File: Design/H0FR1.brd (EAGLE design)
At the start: 60 x 34.6 mm, 34 parts, among them P1 HEXABIT_X2_P1_P5_EDIT_POWER_P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, Q1 BSS123, U1 STM32G0B1CEU6QFN_B1CEU6_STM-L, U2 G5LE-14_DC3, X1 XTALL_CSTCE8M00G52

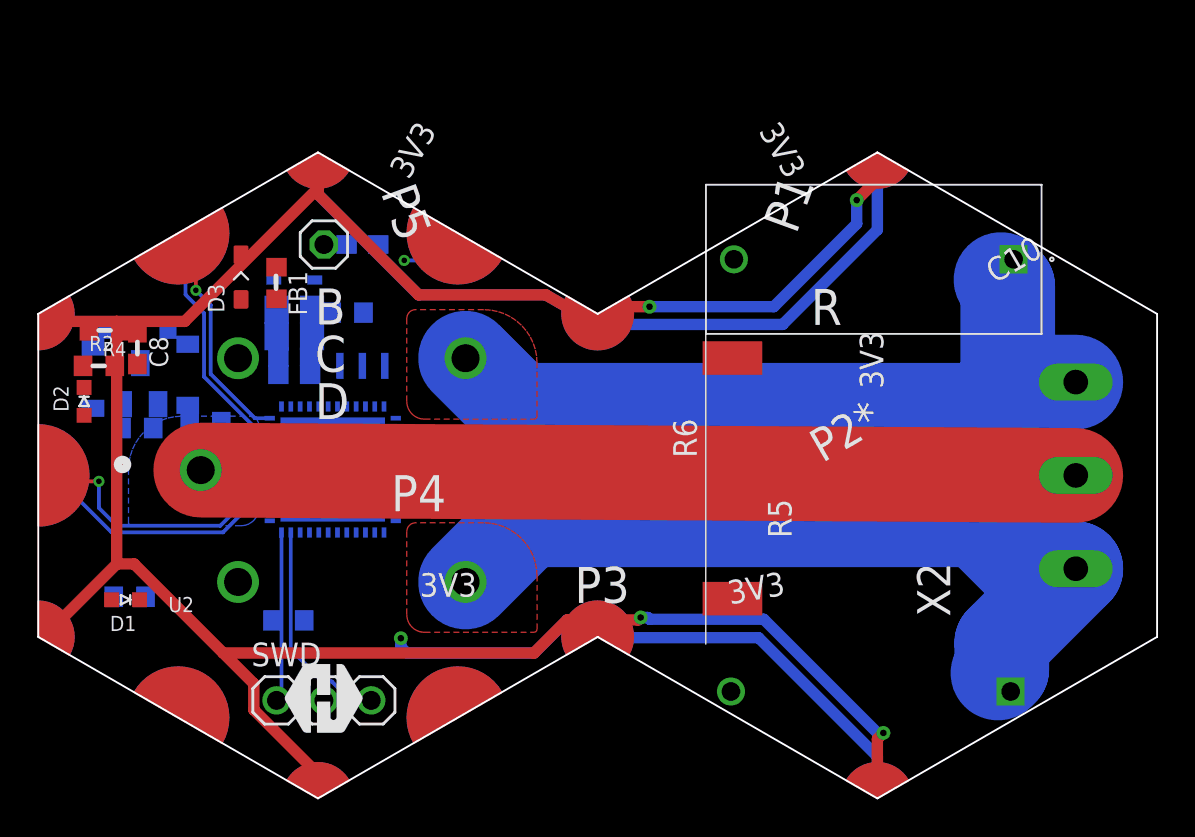
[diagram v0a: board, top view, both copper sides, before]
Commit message: All finish, reviewed version
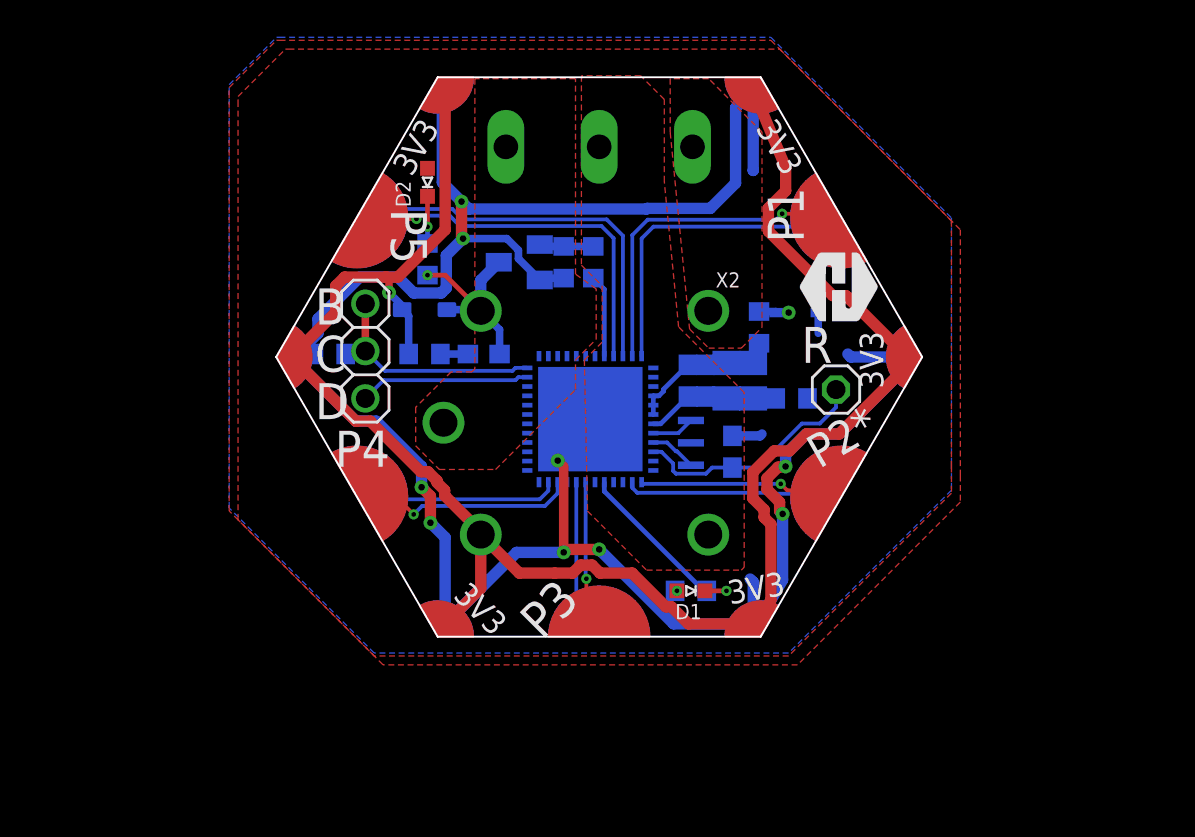
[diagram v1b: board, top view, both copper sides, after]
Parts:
- removed C10, C9: 330nF, HEXABITZ_RCLS:B32922Q_(18_X_8.5)
- removed C2: 1uF, HEXABITZ_RCLS:C-0805
- removed C7: 100nF, HEXABITZ_RCLS:C-0603
- removed D4, D6, D7: MMSZ4705T1GMMSZ4705T1G, HEXABITZ_RCLS:DIO_MMSZ4700T1G
- removed Q1: BSS123, HEXABITZ_RCLS:SOT23
- removed R4: 150, HEXABITZ_RCLS:R-0603
- removed R5, R6: 330, HEXABITZ_RCLS:R2512
- removed TRIMBLE-LOGO2: HEXA-LOGO, HEXABITZ_USER_INTERFACE_PARTS:HEXA-LOGO
- added C3: 100nF, HEXABITZ_RCLS:C-0603
- added C4: 4.7uF, HEXABITZ_RCLS:C-0805
- added Q2: BSS123, HEXABITZ_RCLS:SOT23
- added R10: 150, HEXABITZ_RCLS:R-0603
- added TRIMBLE-LOGO1: HEXA-LOGO, HEXABITZ_USER_INTERFACE_PARTS:HEXA-LOGO
- C1: value 100nF -> 1uF; device HEXABITZ_RCLS:C-0603 -> HEXABITZ_RCLS:C-0805
- C6: value 4.7uF -> 100nF; device HEXABITZ_RCLS:C-0805 -> HEXABITZ_RCLS:C-0603
- D2: value RED -> orange
- FB1: value (none) -> FB-TDK_MMZ1608Y300B
- P1: value HEXABIT_X2_P1_P5_EDIT_POWER_PADS -> HEXABIT_17.32_NO_P6; device hexabitz_connectors:HEXABIT_X2_P1_P5_EDIT_POWER_PADS -> hexabitz_connectors:HEXABIT_17.32_NO_P6
- R2: value 180 -> 180.0 Ω
- R3: value 10k -> 10K
- SWD: device HEXABITZ_CONNECTION_PARTS:SWD -> pinhead:1X03
- moved X2 31.0 mm to (0.00, 26.4), turned to 180 degrees
- moved D1 30.3 mm to (4.92, 2.54)
- moved R1 30.1 mm to (4.92, 2.54), turned to 0 degrees
- moved R 28.5 mm to (12.7, 13.3), turned to 0 degrees
- moved D5 27.0 mm to (10.6, 17.5), turned to 0 degrees
- moved FB1 26.0 mm to (8.57, 16.7), flipped to the bottom, turned to 90 degrees
- moved R8 24.5 mm to (-1.91, 20.2), turned to 270 degrees
- moved R7 24.3 mm to (10.3, 12.9)
- moved C1 23.2 mm to (6.83, 13.8), turned to 270 degrees
- moved R9 22.5 mm to (-0.32, 20.2), turned to 90 degrees
- moved C5 22.1 mm to (5.71, 13.8), turned to 270 degrees
- moved D2 21.8 mm to (-9.21, 24.4), turned to 0 degrees
- moved C6 21.2 mm to (4.76, 13.8), turned to 270 degrees
- moved SWD 18.9 mm to (-12.5, 15.4), turned to 270 degrees
- moved C8 18.6 mm to (-6.19, 15.2), flipped to the bottom, turned to 180 degrees
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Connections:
- removed net COMMON: R5.1, R6.1, U2.1, X2.2
- removed net LED_INDICATOR: D1.A, U1.17
- removed net N$15: C8.2, D3.+, D4.K, Q1.3, R2.1, U2.5
- removed net N$9: C9.2, R5.2
- removed net NORMALLY_CLOSED: C10.1, U2.4, X2.3
- removed net NORMALLY_OPENED: C9.1, U2.3, X2.1
- removed net USART4_RX: U1.12
- removed net USART4_TX: U1.11
- new net COM: U2.1, X2.3
- new net NC: U2.4, X2.1
- new net NO: U2.3, X2.2
- new net USART1_RX: P1.PAD_PD5, U1.46
- new net USART1_TX: P1.PAD_PU5, U1.45
- net GND: now also C3.2, D1.C, D5.1, P1.PAD_PD10, P1.PAD_PD7, P1.PAD_PD8, P1.PAD_PD9, Q2.2; no longer C7.2, D4.A, D5.2, D7.K, P1.PAD_PD13, P1.PAD_PD14, P1.PAD_PD17, P1.PAD_PD18, P1.PAD_PD19, P1.PAD_PD20, Q1.2, R1.2
- net N$1: now also C8.2, D3.+, Q2.3, R2.1, U2.5; no longer D6.A, D7.A
- net N$11: now also Q2.1, R8.1, R9.2; no longer C8.1, R4.1
- net N$12: now also C8.1, R10.1; no longer C10.2, R6.2
- net N$2: now also D1.A, R1.2; no longer D1.C, R1.1
- net N$3: now also R1.1, U1.17; no longer D6.K, Q1.1, R8.1, R9.1
- net N$4: now also C3.1; no longer C7.1
- net RELAY_CONTROL: now also R9.1, U1.44; no longer R9.2, U1.45
- net USART5_RX: now also P1.PAD_PD3, U1.20; no longer P1.PAD_PD5, U1.40
- net USART5_TX: now also P1.PAD_PU3, U1.19; no longer P1.PAD_PU5, U1.41
- net USART6_RX: now also U1.48; no longer P1.PAD_PD3, U1.47
- net USART6_TX: now also U1.47; no longer P1.PAD_PU3, U1.48
- net VDD: now also D5.2, FB1.2, P1.PAD_PU10, P1.PAD_PU7, P1.PAD_PU8, P1.PAD_PU9, R10.2; no longer D5.1, FB1.1, P1.PAD_PU13, P1.PAD_PU14, P1.PAD_PU17, P1.PAD_PU18, P1.PAD_PU19, P1.PAD_PU20, R4.2
- net VDDA: now also C4.1, FB1.1; no longer C2.1, FB1.2
- net VSSA: now also C4.2; no longer C2.2
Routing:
- net GND: track 71.4 -> 131.7 mm, vias 1 -> 10
- net COMMON: track 46.9 -> 0.00 mm
- net NORMALLY_OPENED: track 42.5 -> 0.00 mm
- net NORMALLY_CLOSED: track 40.2 -> 0.00 mm
- net VDD: track 132.6 -> 101.1 mm, vias 4 -> 2
- net USART1_RX: track 0.00 -> 21.0 mm
- net USART1_TX: track 0.00 -> 20.2 mm, vias 0 -> 1
- net N$4: track 0.00 -> 12.9 mm
- net USART3_TX: track 0.00 -> 11.8 mm, vias 0 -> 1
- net N$1: track 0.00 -> 11.4 mm, vias 0 -> 1
- net USART3_RX: track 0.00 -> 10.8 mm
- net USART2_TX: track 0.00 -> 10.3 mm, vias 0 -> 1
- net VDDA: track 0.00 -> 8.33 mm
- net USART2_RX: track 2.88 -> 11.1 mm, vias 1 -> 0
- net N$3: track 0.00 -> 8.20 mm
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- added copper zone on layer 1, net COM
- added copper zone on layer 16, net GND
- added copper zone on layer 1, net NC
- added copper zone on layer 1, net NO
- removed copper zone on layer 16, net VDD
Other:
- board size 60 x 34.6 mm -> 34.6 x 30 mm
- board text added: "230V/10A (RMS)"
- board text added: "COM"
- board text added: "NC"
- board text added: "NO"
- board text removed: "30VDC/4A"
